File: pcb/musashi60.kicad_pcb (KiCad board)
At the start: 2 copper layers, 185 x 130 mm, 74 parts, among them J1 MJ-4PP-9, U1 ProMicro_r

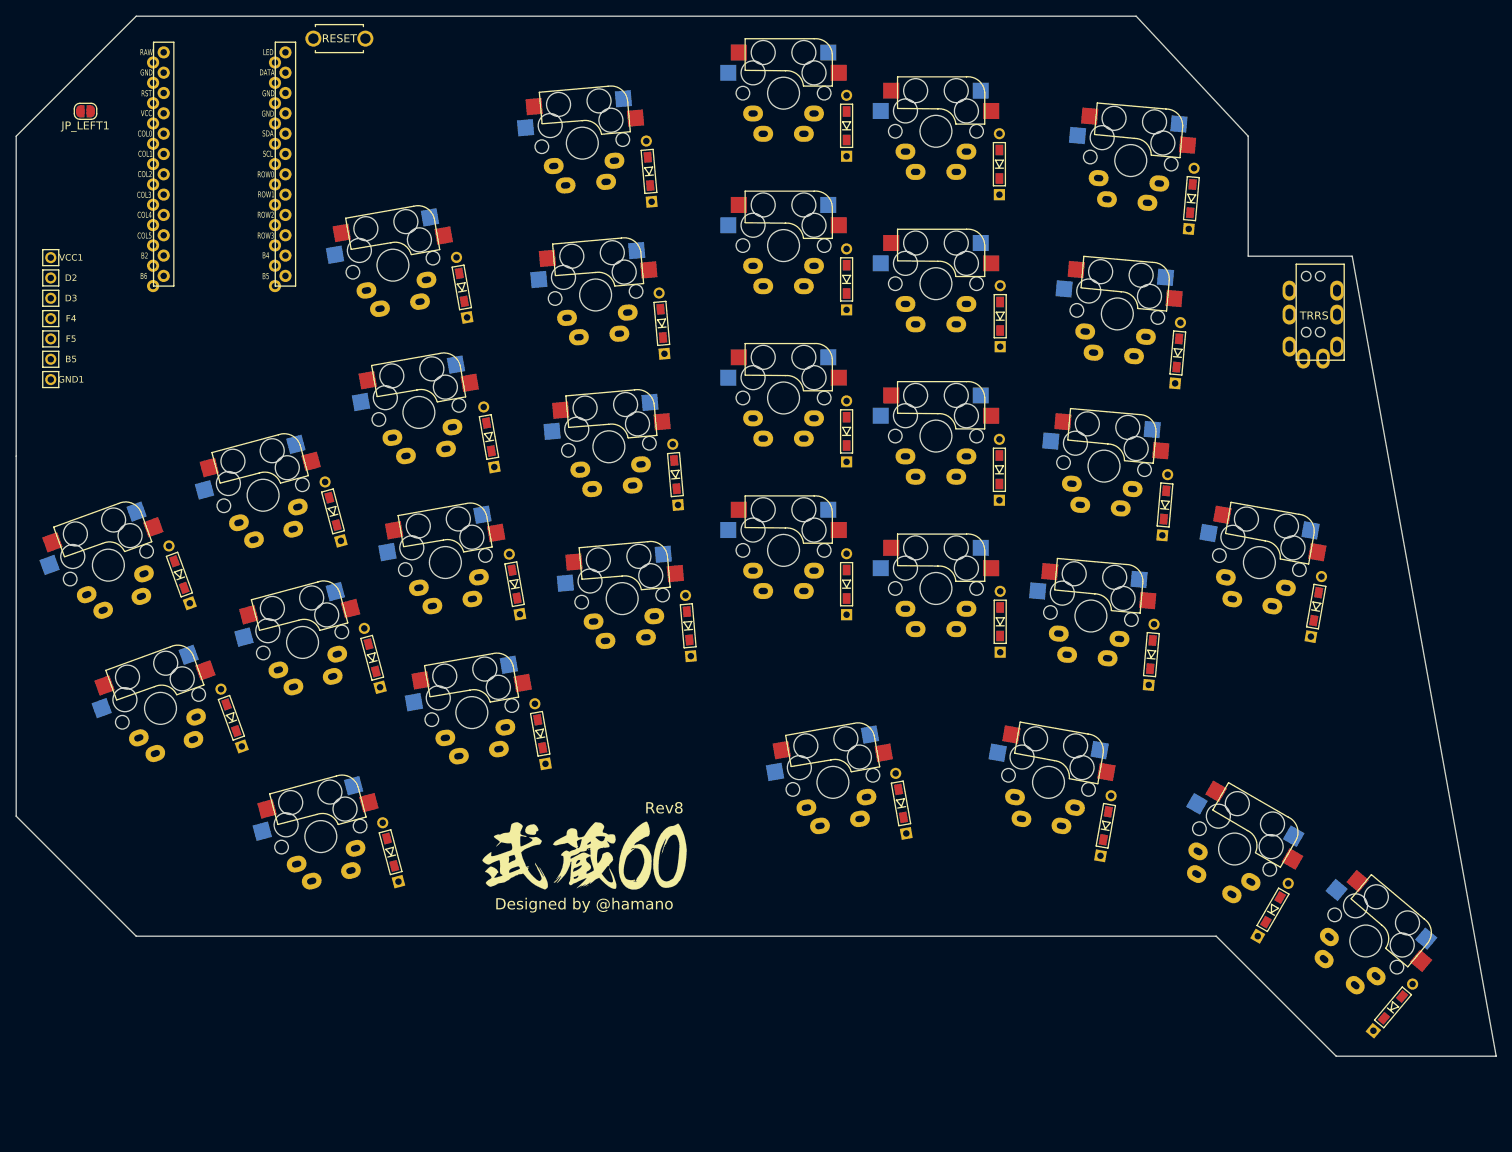
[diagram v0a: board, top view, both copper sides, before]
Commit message: update pcb for rev8
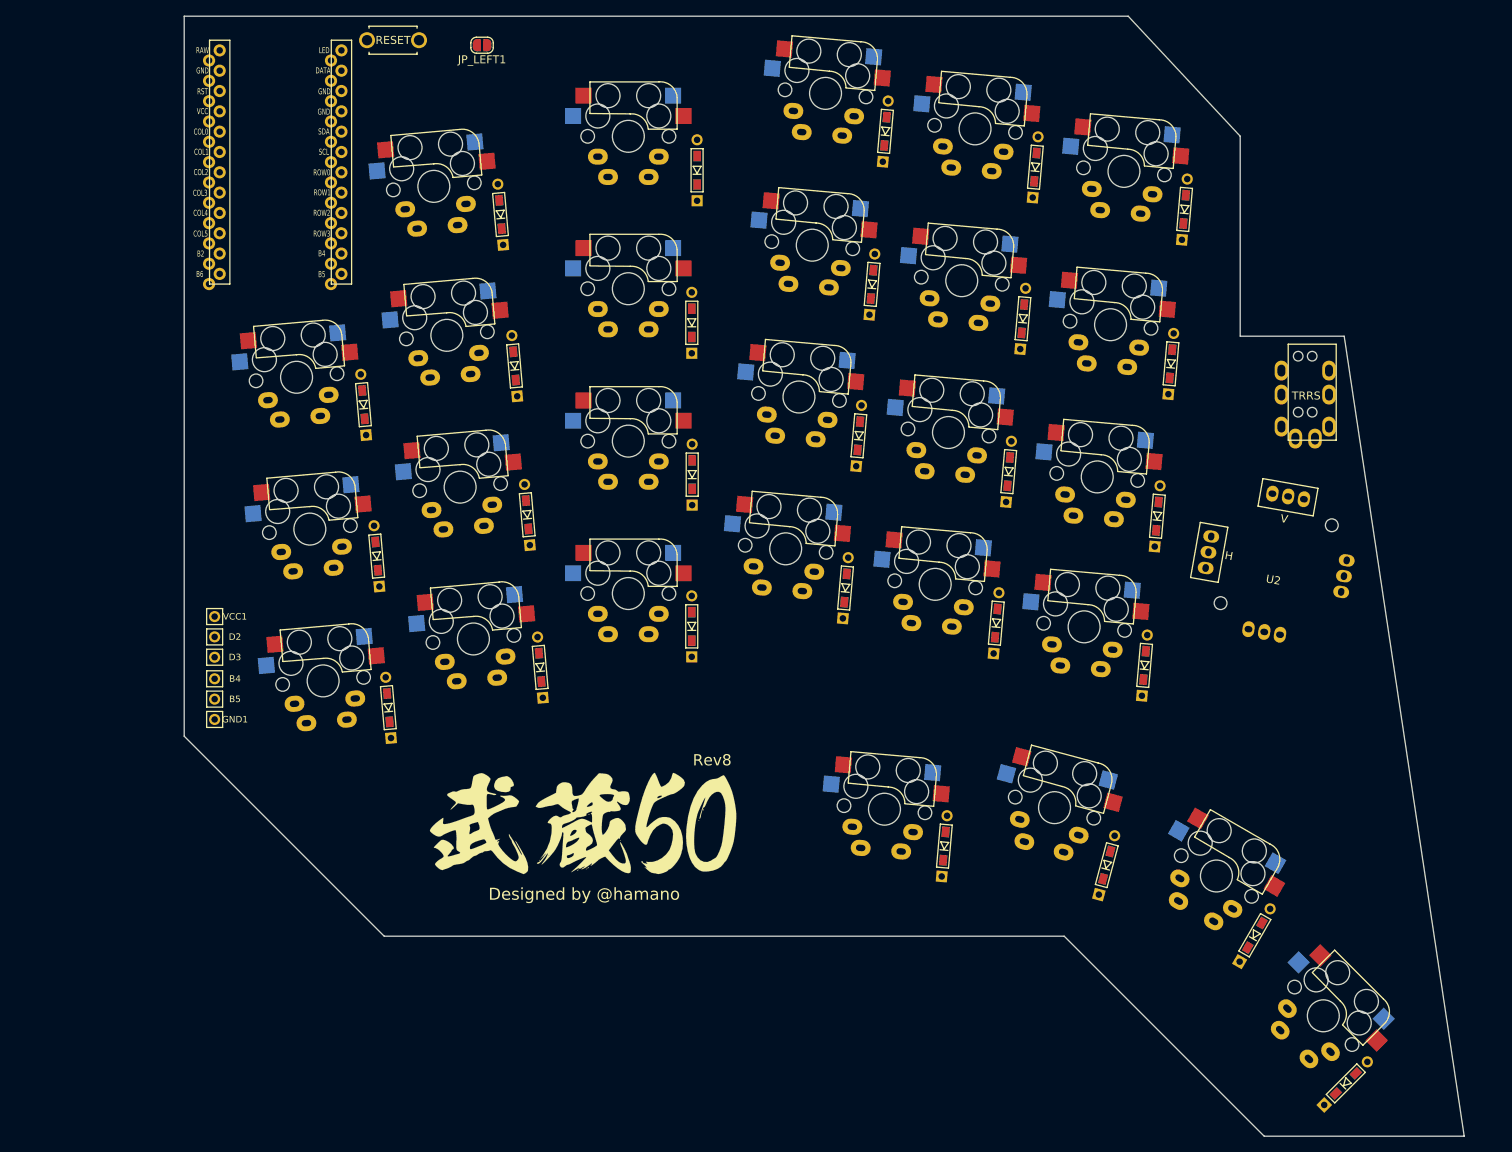
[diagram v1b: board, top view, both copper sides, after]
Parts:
- removed the D_A5 at (178.5, 86.8)
- removed D_F5, D_G3: D, foostan:D3_TH_SMD
- removed F4: MountingHole_Pad, foostan:1pin_conn
- removed the G_LOGO_B at (87.0, 118.0)
- removed the G_LOGO_F at (87.0, 118.0)
- removed the SW_A5 at (171.4, 81.3)
- removed SW_F5, SW_G3: SW_PUSH, local:CherryMX_Direct_Hotswap_Reversible
- added G_LOGO_B: LOGO, local:musashi50-silk-256, B.Cu at (87.0, 113.0)
- added G_LOGO_F: LOGO, local:musashi50-silk-256, F.Cu at (87.0, 113.0)
- added U2: joystick, local:J08K, F.Cu at (173.5, 81.5)
- moved JP_LEFT1 50.2 mm to (74.2, 16.6)
- moved JP_RIGHT1 50.2 mm to (74.2, 16.6)
- moved D3 49.3 mm to (40.8, 93.1)
- moved VCC1 49.3 mm to (40.8, 88.0)
- moved D2 49.3 mm to (40.8, 90.6)
- moved B4 47.2 mm to (40.8, 95.8)
- moved GND1 47.2 mm to (40.8, 100.9)
- moved B5 47.2 mm to (40.8, 98.4)
- moved SW_F2 33.2 mm to (51.0, 58.1), turned to 5 degrees
- moved D_F2 31.3 mm to (59.4, 61.6), turned to 95 degrees
- moved D_A5 11.2 mm to (182.2, 146.4), turned to 45 degrees
- moved SW_E1 11.1 mm to (68.2, 34.3), turned to 5 degrees
- moved SW_A5 10.8 mm to (179.4, 138.0), turned to 315 degrees
- moved D_E1 10.3 mm to (76.5, 37.8), turned to 95 degrees
- moved SW_E2 10.3 mm to (69.8, 52.9), turned to 5 degrees
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- renumbered F5 to B4, D_B5 to D_A5, D_C5 to D_B5, D_D5 to D_C5, D_E5 to D_D5, D_G2 to D_F2, D_F2 to D_F3, D_F3 to D_F4, SW_B5 to SW_A5, SW_C5 to SW_B5, SW_D5 to SW_C5, SW_E5 to SW_D5, SW_G2 to SW_F2, SW_F2 to SW_F3, SW_F3 to SW_F4
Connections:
- B4 pad 1: F5 -> B4
- D_F3 pad 1: F7 -> B1
- D_F4 pad 1: B1 -> B3
- SW_A5 pad 1: D0 -> D1
- SW_B5 pad 1: D4 -> D0
- SW_C5 pad 1: C6 -> D4
- SW_D5 pad 1: D7 -> C6
- SW_F2 pad 1: B4 -> E6
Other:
- board size 185 x 130 mm -> 160 x 140 mm
